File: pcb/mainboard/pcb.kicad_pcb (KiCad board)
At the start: 4 copper layers, 60 x 60 mm, 268 parts, among them J1 USB_C_Receptacle, J2 DNP, J3 FH12-40S-0.5SH, J4 DVI, J5 SM03B-SRSS-TB, Q1 AO3401A, Q2 S8050, Q6 AO3400A, Q7 AO3401A, Q8 AO3401A, SW1 SW, SW2 SW, U1 SY8120, U10 LGS5148, U11 LM321, U12 MT41K64M16TW, U13 W25Q32JV, U14 RP2040, U15 ADV7611, U16 USBLC6-2P6, U17 FUSB302BMPX, U18 CBTL02043A, U19 PTN3460, U2 SY8120, U3 SY8120, U4 MT9700, U5 XC6SLX16-FTG256, U6 MT9700, U7 MT3608(SOT23-6), U8 MT3608(SOT23-6), U9 LGS5148, Y1 33MHz, Y2 12MHz, Y3 28.63636MHz

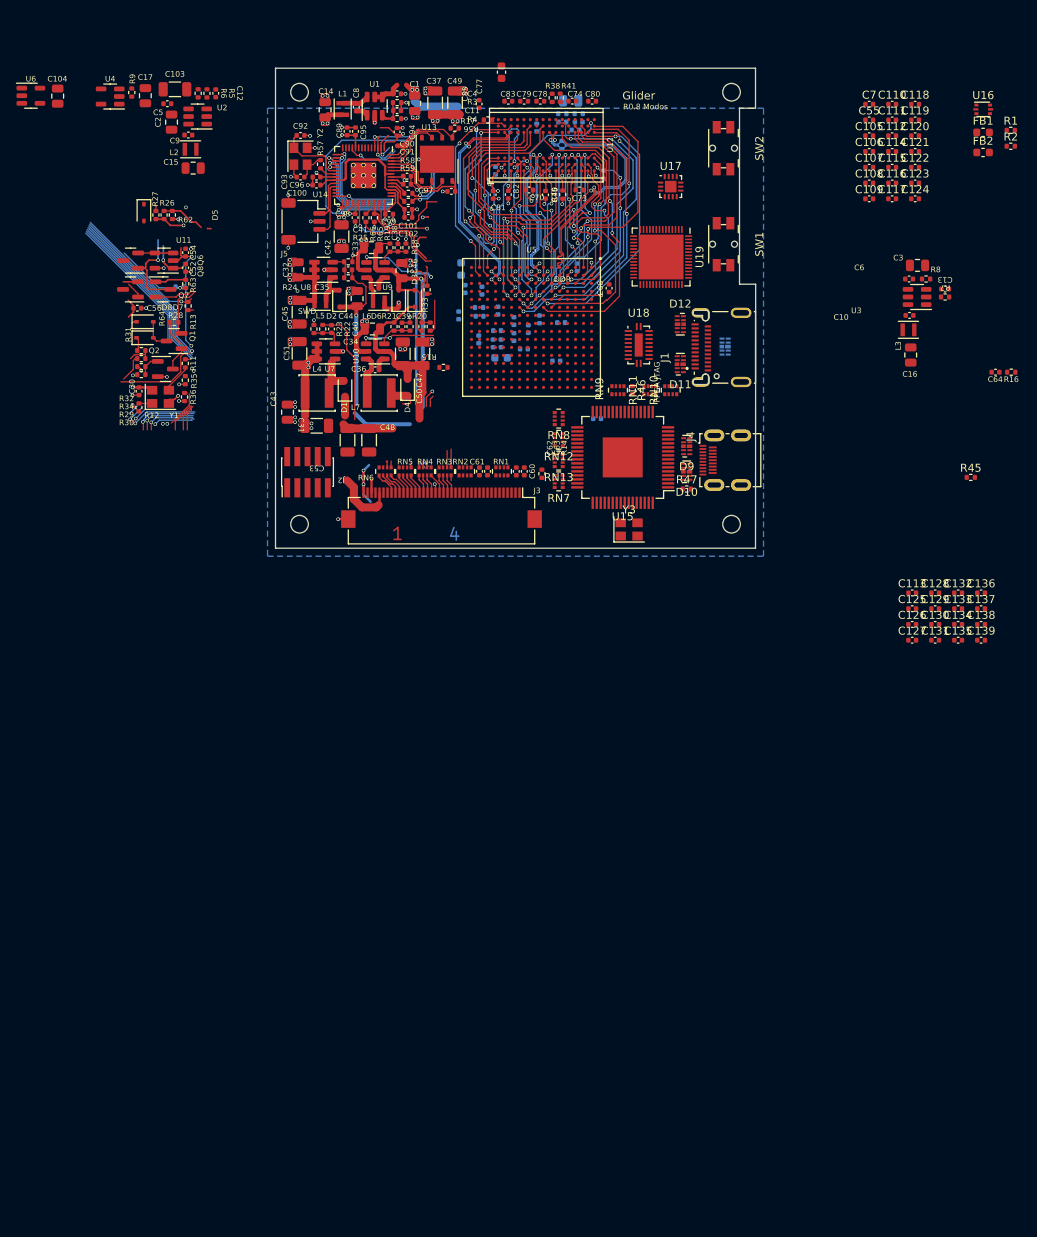
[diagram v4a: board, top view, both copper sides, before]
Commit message: r0p7 wip
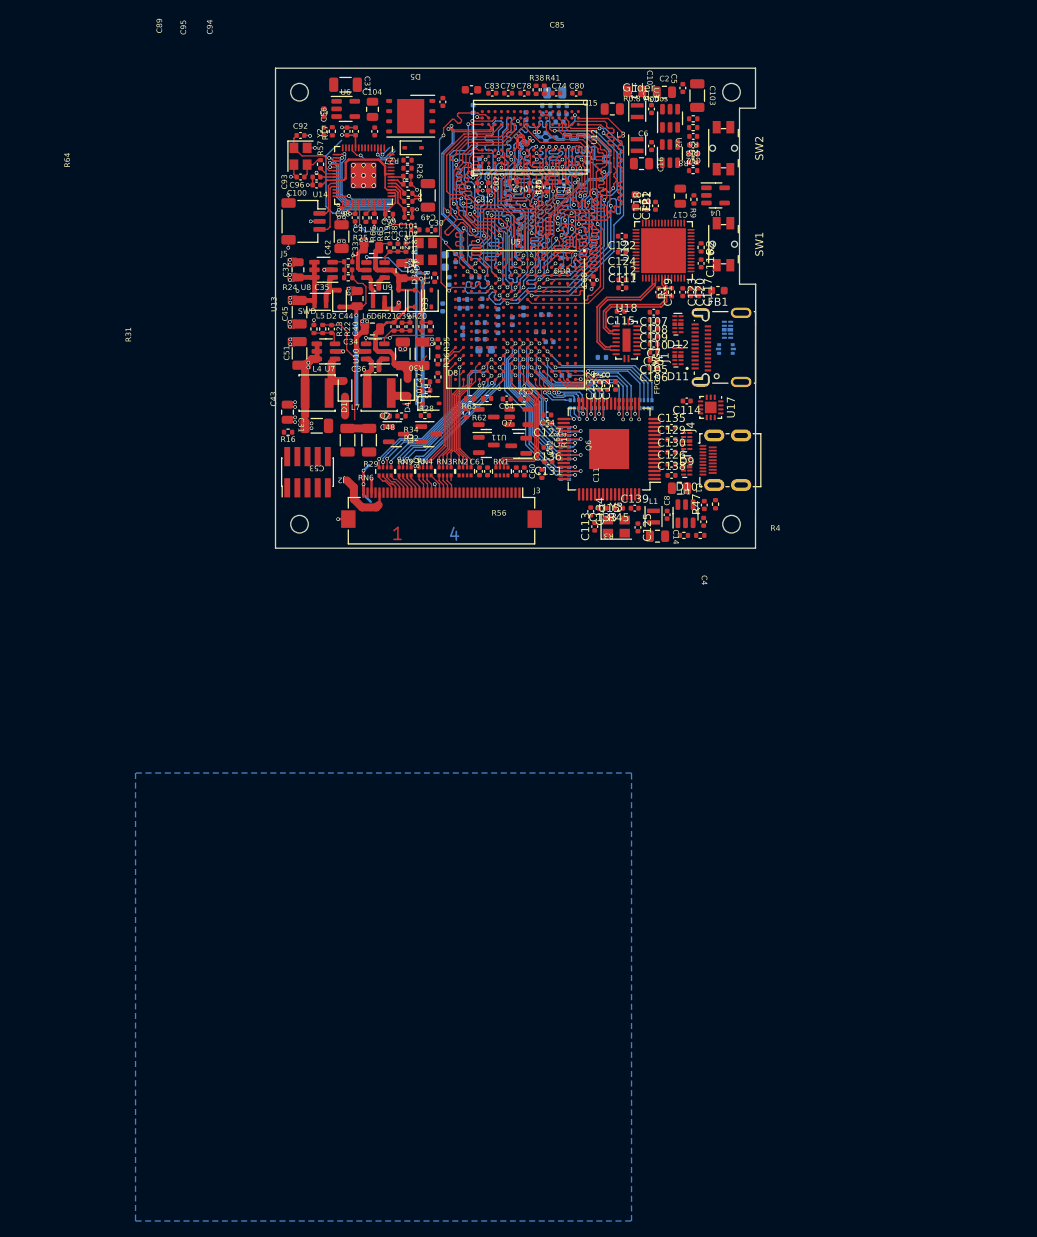
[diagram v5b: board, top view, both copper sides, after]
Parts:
- removed R10: 4.7K, Resistor_SMD:R_0402_1005Metric
- C77, R13, R46, RN10, RN11, RN12, RN13, RN7, RN8, RN9, U16: moved to B.Cu
- moved R16 90.7 mm to (96.6, 85.5)
- moved U4 76.7 mm to (150.0, 55.9), turned to 0 degrees
- moved R9 71.5 mm to (147.3, 56.4), turned to -90 degrees
- moved C17 68.0 mm to (145.6, 56.0), turned to 90 degrees
- moved C14 67.6 mm to (142.8, 98.5), turned to 180 degrees
- moved C103 65.3 mm to (147.7, 43.4), turned to 90 degrees
- moved R3 64.9 mm to (146.1, 98.4), turned to 180 degrees
- moved C5 64.5 mm to (145.9, 42.5), turned to -90 degrees
- moved R4 64.4 mm to (148.1, 98.4)
- moved C4 64.2 mm to (148.6, 94.6), turned to 90 degrees
- moved C11 64.1 mm to (148.5, 96.7), turned to 90 degrees
- moved C8 64.1 mm to (143.9, 95.8)
- moved L1 64.1 mm to (142.2, 96.0)
- moved U1 64.1 mm to (146.2, 95.7)
- moved R6 62.0 mm to (147.2, 46.3), turned to 180 degrees
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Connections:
- RN10 pad 5: DPI_R7 -> DPI_R4
- RN10 pad 6: DPI_R6 -> DPI_R5
- RN10 pad 7: DPI_R5 -> DPI_R6
- RN10 pad 8: DPI_R4 -> DPI_R7
- RN11 pad 5: DPI_R3 -> DPI_R0
- RN11 pad 6: DPI_R2 -> DPI_R1
- RN11 pad 7: DPI_R1 -> DPI_R2
- RN11 pad 8: DPI_R0 -> DPI_R3
- RN12 pad 5: DPI_B7 -> DPI_B4
- RN12 pad 6: DPI_B6 -> DPI_B5
- RN12 pad 7: DPI_B5 -> DPI_B6
- RN12 pad 8: DPI_B4 -> DPI_B7
- RN13 pad 5: DPI_B3 -> DPI_B0
- RN13 pad 6: DPI_B2 -> DPI_B1
- RN13 pad 7: DPI_B1 -> DPI_B2
- RN13 pad 8: DPI_B0 -> DPI_B3
- RN7 pad 6: DPI_DE -> DPI_VS
- RN7 pad 8: DPI_VS -> DPI_DE
- RN8 pad 5: DPI_G3 -> DPI_G0
- RN8 pad 6: DPI_G2 -> DPI_G1
- RN8 pad 7: DPI_G1 -> DPI_G2
- RN8 pad 8: DPI_G0 -> DPI_G3
- RN9 pad 5: DPI_G7 -> DPI_G4
- RN9 pad 6: DPI_G6 -> DPI_G5
- RN9 pad 7: DPI_G5 -> DPI_G6
- RN9 pad 8: DPI_G4 -> DPI_G7
- U15 pad 15: Net-(RN10-R4.1) -> Net-(RN10-R1.1)
- U15 pad 16: Net-(RN10-R3.1) -> Net-(RN10-R2.1)
- U15 pad 17: Net-(RN10-R2.1) -> Net-(RN10-R3.1)
- U15 pad 18: Net-(RN10-R1.1) -> Net-(RN10-R4.1)
- U15 pad 19: Net-(RN11-R4.1) -> Net-(RN11-R1.1)
- U15 pad 20: Net-(RN11-R3.1) -> Net-(RN11-R2.1)
- U15 pad 21: Net-(RN11-R2.1) -> Net-(RN11-R3.1)
- U15 pad 22: Net-(RN11-R1.1) -> Net-(RN11-R4.1)
- U15 pad 26: Net-(RN9-R4.1) -> Net-(RN9-R1.1)
- U15 pad 27: Net-(RN9-R3.1) -> Net-(RN9-R2.1)
- U15 pad 28: Net-(RN9-R2.1) -> Net-(RN9-R3.1)
- U15 pad 29: Net-(RN9-R1.1) -> Net-(RN9-R4.1)
- U15 pad 30: Net-(RN8-R4.1) -> Net-(RN8-R1.1)
- U15 pad 31: Net-(RN8-R3.1) -> Net-(RN8-R2.1)
- U15 pad 32: Net-(RN8-R2.1) -> Net-(RN8-R3.1)
- U15 pad 33: Net-(RN8-R1.1) -> Net-(RN8-R4.1)
- U15 pad 35: Net-(RN12-R4.1) -> Net-(RN12-R1.1)
- U15 pad 36: Net-(RN12-R3.1) -> Net-(RN12-R2.1)
- U15 pad 37: Net-(RN12-R2.1) -> Net-(RN12-R3.1)
- U15 pad 38: Net-(RN12-R1.1) -> Net-(RN12-R4.1)
- U15 pad 39: Net-(RN13-R4.1) -> Net-(RN13-R1.1)
- U15 pad 41: Net-(RN13-R3.1) -> Net-(RN13-R2.1)
- U15 pad 42: Net-(RN13-R2.1) -> Net-(RN13-R3.1)
- U15 pad 43: Net-(RN13-R1.1) -> Net-(RN13-R4.1)
- U15 pad 45: Net-(RN7-R3.1) -> Net-(RN7-R1.1)
- U15 pad 47: Net-(RN7-R1.1) -> Net-(RN7-R3.1)
- U18 pad 11: GND -> Net-(U18-GND-Pad11)
- U18 pad 12: /dp_in/RX2PC -> /dp_in/RX1PC
- U18 pad 13: /dp_in/RX2NC -> /dp_in/RX1NC
- U18 pad 14: /dp_in/TX2PC -> /dp_in/TX1PC
- U18 pad 15: /dp_in/TX2NC -> /dp_in/TX1NC
- U18 pad 16: /dp_in/RX1PC -> /dp_in/RX2PC
- U18 pad 17: /dp_in/RX1NC -> /dp_in/RX2NC
- U18 pad 18: /dp_in/TX1PC -> /dp_in/TX2PC
- U18 pad 19: /dp_in/TX1NC -> /dp_in/TX2NC
- U18 pad 20: GND -> Net-(U18-GND-Pad11)
- U18 pad 21: GND -> Net-(U18-GND-Pad11)
- U18 pad 5: GND -> Net-(U18-GND-Pad11)
- U5 pad A10: unconnected-(U5A-IO_L35N_GCLK16_0-PadA10) -> LVDS_ODD_CKN
- U5 pad A13: unconnected-(U5A-IO_L63N_SCP6_0-PadA13) -> LVDS_EVEN_CN
- U5 pad A6: TMDS_D2P -> unconnected-(U5A-IO_L4N_0-PadA6)
- U5 pad A8: unconnected-(U5A-IO_L33N_0-PadA8) -> LVDS_ODD_CN
- U5 pad A9: TMDS_D0P -> unconnected-(U5A-IO_L34N_GCLK18_0-PadA9)
- U5 pad B10: unconnected-(U5A-IO_L35P_GCLK17_0-PadB10) -> LVDS_ODD_CKP
- U5 pad B15: unconnected-(U5A-IO_L29P_A23_M1A13_1-PadB15) -> DPI_R5
- U5 pad B16: unconnected-(U5A-IO_L29N_A22_M1A14_1-PadB16) -> DPI_R4
- U5 pad B6: TMDS_D2N -> unconnected-(U5A-IO_L4P_0-PadB6)
- U5 pad B8: unconnected-(U5A-IO_L33P_0-PadB8) -> LVDS_ODD_CP
- U5 pad C10: TMDS_CKP -> unconnected-(U5A-IO_L37N_GCLK12_0-PadC10)
- U5 pad C13: unconnected-(U5A-IO_L63P_SCP7_0-PadC13) -> LVDS_EVEN_CP
- U5 pad C15: unconnected-(U5A-IO_L33P_A15_M1A10_1-PadC15) -> DPI_R3
- U5 pad C16: unconnected-(U5A-IO_L33N_A14_M1A4_1-PadC16) -> DPI_R2
- U5 pad C4: Net-(U5A-IO_L1P_HSWAPEN_0) -> unconnected-(U5A-IO_L1P_HSWAPEN_0-PadC4)
- U5 pad C5: unconnected-(U5A-IO_L3N_0-PadC5) -> LVDS_ODD_AN
- U5 pad C6: TMDS_D1P -> unconnected-(U5A-IO_L7N_0-PadC6)
- U5 pad C9: TMDS_D0N -> unconnected-(U5A-IO_L34P_GCLK19_0-PadC9)
- U5 pad D14: unconnected-(U5A-IO_L31P_A19_M1CKE_1-PadD14) -> DPI_R6
- U5 pad D16: unconnected-(U5A-IO_L31N_A18_M1A12_1-PadD16) -> DPI_G3
- U5 pad D5: unconnected-(U5A-IO_L3P_0-PadD5) -> LVDS_ODD_AP
- U5 pad D6: TMDS_D1N -> unconnected-(U5A-IO_L7P_0-PadD6)
- U5 pad D9: unconnected-(U5A-IO_L40N_0-PadD9) -> LVDS_EVEN_BN
- U5 pad E10: TMDS_CKN -> unconnected-(U5A-IO_L37P_GCLK13_0-PadE10)
- U5 pad E12: unconnected-(U5A-IO_L1N_A24_VREF_1-PadE12) -> DPI_R7
- U5 pad E13: unconnected-(U5A-IO_L1P_A25_1-PadE13) -> DPI_R1
- U5 pad E15: unconnected-(U5A-IO_L34P_A13_M1WE_1-PadE15) -> DPI_G2
- U5 pad E16: unconnected-(U5A-IO_L34N_A12_M1BA2_1-PadE16) -> DPI_G1
- U5 pad E6: unconnected-(U5A-IO_L5N_0-PadE6) -> LVDS_ODD_BN
- U5 pad E7: unconnected-(U5A-IO_L36P_GCLK15_0-PadE7) -> LVDS_EVEN_AP
- U5 pad E8: unconnected-(U5A-IO_L36N_GCLK14_0-PadE8) -> LVDS_EVEN_AN
- U5 pad F12: unconnected-(U5A-IO_L30P_A21_M1RESET_1-PadF12) -> DPI_G6
- U5 pad F13: unconnected-(U5A-IO_L32P_A17_M1A8_1-PadF13) -> DPI_R0
- U5 pad F14: unconnected-(U5A-IO_L32N_A16_M1A9_1-PadF14) -> DPI_G7
- U5 pad F15: unconnected-(U5A-IO_L35P_A11_M1A7_1-PadF15) -> DPI_G0
- U5 pad F16: unconnected-(U5A-IO_L35N_A10_M1A2_1-PadF16) -> DPI_B7
- U5 pad F7: unconnected-(U5A-IO_L5P_0-PadF7) -> LVDS_ODD_BP
- U5 pad F9: unconnected-(U5A-IO_L40P_0-PadF9) -> LVDS_EVEN_BP
- U5 pad G11: unconnected-(U5A-IO_L30N_A20_M1A11_1-PadG11) -> DPI_B6
- U5 pad G12: unconnected-(U5A-IO_L38P_A5_M1CLK_1-PadG12) -> DPI_G4
- U5 pad G14: unconnected-(U5A-IO_L36P_A9_M1BA0_1-PadG14) -> DPI_G5
- U5 pad H11: unconnected-(U5A-IO_L38N_A4_M1CLKN_1-PadH11) -> DPI_B2
- U5 pad H13: unconnected-(U5A-IO_L39P_M1A3_1-PadH13) -> DPI_B3
- U5 pad H14: unconnected-(U5A-IO_L39N_M1ODT_1-PadH14) -> DPI_B5
- U5 pad H15: unconnected-(U5A-IO_L37P_A7_M1A0_1-PadH15) -> DPI_B4
- U5 pad J11: unconnected-(U5A-IO_L40P_GCLK11_M1A5_1-PadJ11) -> DPI_HS
- U5 pad J12: unconnected-(U5A-IO_L40N_GCLK10_M1A6_1-PadJ12) -> DPI_DE
- U5 pad J13: unconnected-(U5A-IO_L41P_GCLK9_IRDY1_M1RASN_1-PadJ13) -> DPI_B0
- U5 pad J14: EPDC_D10 -> DPI_B1
- U5 pad K11: unconnected-(U5A-IO_L42N_GCLK6_TRDY1_M1LDM_1-PadK11) -> DPI_PCLK
- U5 pad K12: unconnected-(U5A-IO_L42P_GCLK7_M1UDM_1-PadK12) -> DPI_VS
- U5 pad K14: unconnected-(U5A-IO_L41N_GCLK8_M1CASN_1-PadK14) -> EPDC_D10
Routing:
- net VNEG: track 85.1 -> 20.7 mm, vias 3 -> 0
- net +DRAM_VREF: track 2.64 -> 38.2 mm, vias 0 -> 4
- net FPGA_MOSI: track 34.5 -> 12.9 mm
- net FPGA_SCLK: track 35.0 -> 13.4 mm
- net FPGA_CS: track 33.8 -> 12.4 mm
- net +3V3: track 51.4 -> 30.6 mm, vias 17 -> 14
- net /fpga_ddr/DRAM_WEB: track 15.2 -> 35.9 mm
- net +5V: track 20.3 -> 0.00 mm, vias 2 -> 0
- net DPI_HS: track 0.00 -> 20.3 mm, vias 0 -> 1
- net /fpga_ddr/DRAM_BA2: track 15.9 -> 35.9 mm
- net DPI_VS: track 0.00 -> 19.6 mm, vias 0 -> 1
- net DPI_DE: track 0.00 -> 18.7 mm, vias 0 -> 1
- net EPDC_SDCE0: track 3.27 -> 21.9 mm, vias 1 -> 2
- net /fpga_ddr/DRAM_ADDR2: track 16.7 -> 35.2 mm
- net /fpga_ddr/DRAM_ADDR9: track 17.5 -> 35.9 mm
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- removed copper zone on F.Cu, net +3V3
- removed copper zone on F.Cu, net +5V
- removed copper zone on In2.Cu, net +5V_EPD
